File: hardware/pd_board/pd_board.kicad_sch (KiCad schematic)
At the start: 48 parts, among them J1 USB_C_Receptacle_USB2.0_16P, J2 CC1_TP, J3 CC2_TP, J4 Debug Port, J5 UART_Port, J6 VBUS_JP, J7 VCONN_JP, J8 VIN_ENA_JP, U1 FUSB302BMPX, U2 TPS5420D, U3 STM32F072CBUx

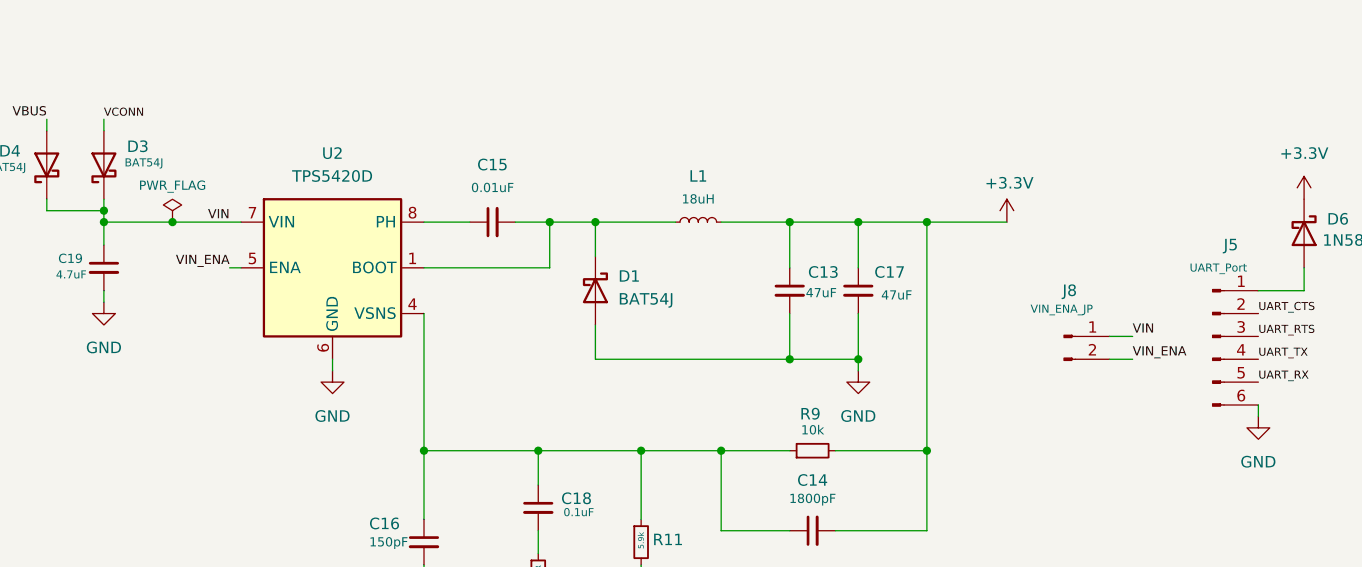
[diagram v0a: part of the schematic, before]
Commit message: update
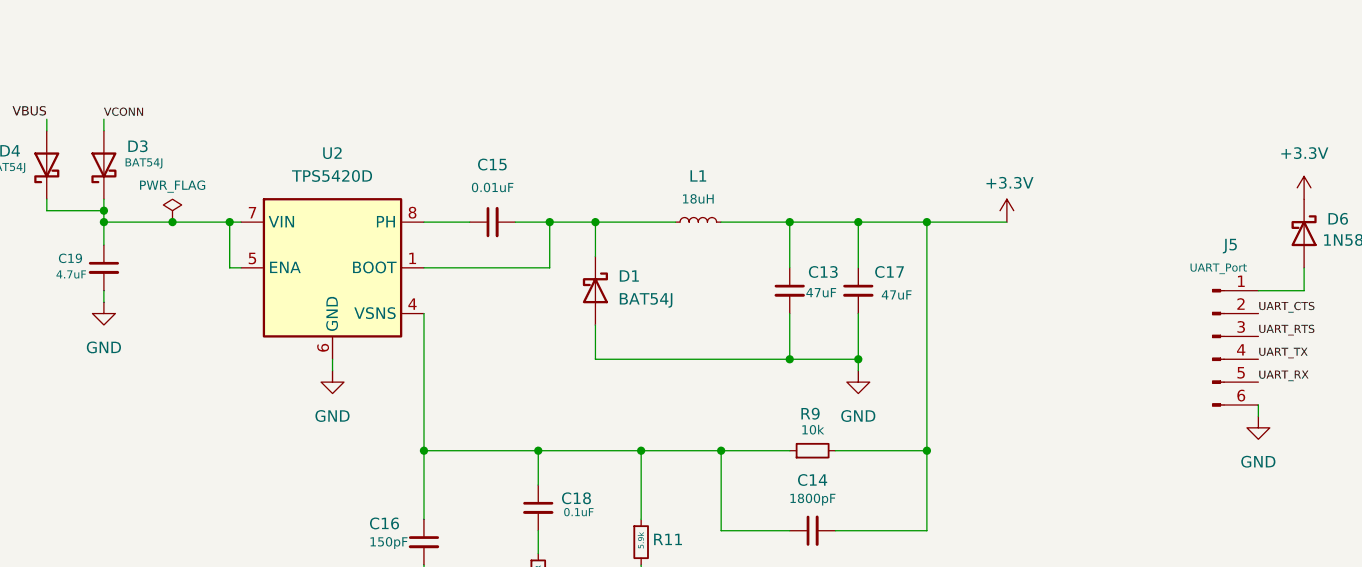
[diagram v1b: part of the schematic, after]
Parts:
- removed J8: VIN_ENA_JP, Connector_PinHeader_2.54mm:PinHeader_1x02_P2.54mm_Vertical, symbol Connector:Conn_01x02_Pin
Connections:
- net VIN_ENA is gone; now on an unnamed net: U2.5 (ENA)
- net VIN: no longer names the net of C19.1, D3.1 (K), D4.1 (K), U2.7 (VIN)

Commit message: update
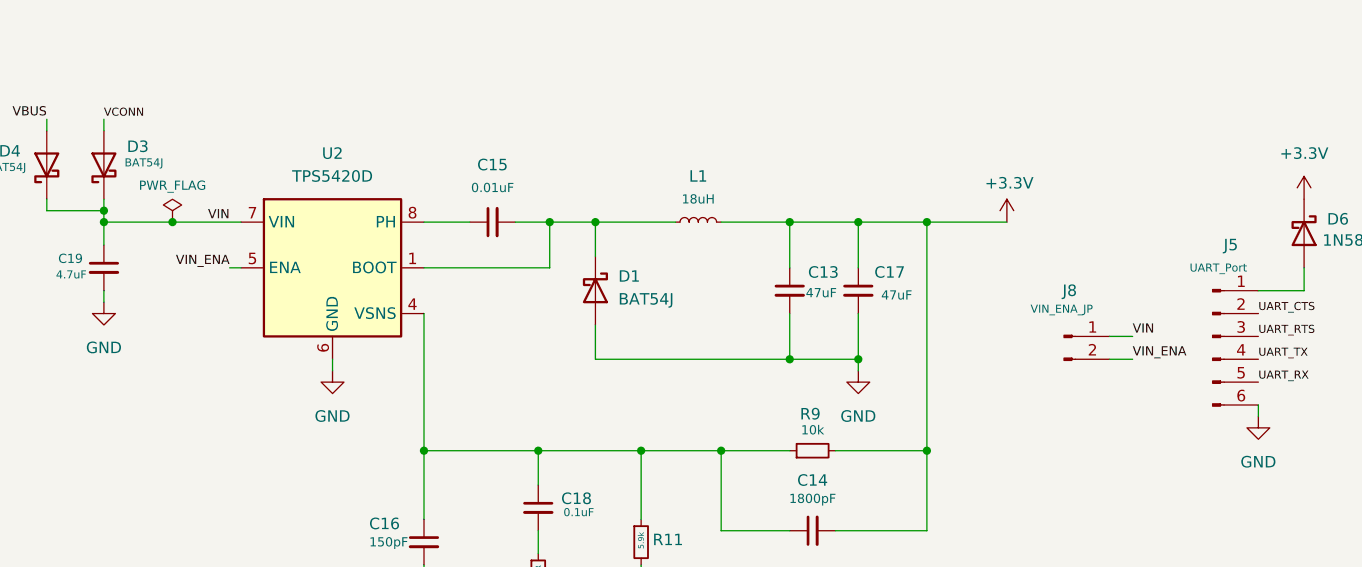
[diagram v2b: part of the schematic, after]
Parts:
- added J8: VIN_ENA_JP, Connector_PinHeader_2.54mm:PinHeader_1x02_P2.54mm_Vertical, symbol Connector:Conn_01x02_Pin
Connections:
- net VIN: now reaches C19.1, D3.1 (K), D4.1 (K), U2.7 (VIN)
- net VIN: now also J8.1 (Pin_1); no longer U2.5 (ENA)
- new net VIN_ENA: J8.2 (Pin_2), U2.5 (ENA)
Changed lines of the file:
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@@
-	)
-	(junction
-		(at 48.26 121.92)
-		(diameter 0)
-		(color 0 0 0 0)
 	)
 	(junction
@@
 	(wire
 		(pts
+			(xy 146.05 137.16) (xy 148.59 137.16)
+		)
+		(stroke
+			(width 0)
+			(type default)
+		)
+	)
+	(wire
+		(pts
 			(xy 27.94 110.49) (xy 27.94 111.76)
 		)
@@
 	(wire
 		(pts
-			(xy 48.26 121.92) (xy 49.53 121.92)
-		)
-		(stroke
-			(width 0)
-			(type default)
-		)
-	)
-	(wire
-		(pts
 			(xy 82.55 40.64) (xy 110.49 40.64)
 		)
@@
 	(wire
 		(pts
+			(xy 49.53 127) (xy 48.26 127)
+		)
+		(stroke
+			(width 0)
+			(type default)
+		)
+	)
+	(wire
+		(pts
 			(xy 175.26 27.94) (xy 177.8 27.94)
 		)
@@
 	(wire
 		(pts
-			(xy 48.26 127) (xy 48.26 121.92)
-		)
-		(stroke
-			(width 0)
-			(type default)
-		)
-	)
-	(wire
-		(pts
-			(xy 49.53 127) (xy 48.26 127)
-		)
-		(stroke
-			(width 0)
-			(type default)
-		)
-	)
-	(wire
-		(pts
 			(xy 82.55 167.64) (xy 93.98 167.64)
 		)
@@
 	(wire
 		(pts
+			(xy 146.05 134.62) (xy 148.59 134.62)
+		)
+		(stroke
+			(width 0)
+			(type default)
+		)
+	)
+	(wire
+		(pts
 			(xy 102.87 147.32) (xy 110.49 147.32)
 		)
@@
 	(wire
 		(pts
-			(xy 41.91 121.92) (xy 48.26 121.92)
+			(xy 41.91 121.92) (xy 49.53 121.92)
 		)
 		(stroke
@@
 		)
 	)
+	(label "VIN"
+		(at 148.59 134.62 0)
+		(effects
+			(font
+				(size 1.016 1.016)
+			)
+			(justify left bottom)
+		)
+	)
 	(label "I2C_SDA"
 		(at 205.74 95.25 180)
@@
 		)
 	)
+	(label "VIN"
+		(at 48.26 121.92 180)
+		(effects
+			(font
+				(size 1.016 1.016)
+			)
+			(justify right bottom)
+		)
+	)
 	(label "VBUS"
 		(at 27.94 110.49 180)
@@
 		)
 	)
+	(label "VIN_ENA"
+		(at 148.59 137.16 0)
+		(effects
+			(font
+				(size 1.016 1.016)
+			)
+			(justify left bottom)
+		)
+	)
 	(label "VBUS"
 		(at 111.76 36.83 0)
@@
 			)
 			(justify left bottom)
+		)
+	)
+	(label "VIN_ENA"
+		(at 48.26 127 180)
+		(effects
+			(font
+				(size 1.016 1.016)
+			)
+			(justify right bottom)
 		)
 	)
@@
 					(unit 1)
 				)
+			)
+		)
+	)
+	(symbol
+		(lib_id "Connector:Conn_01x02_Pin")
+		(at 140.97 134.62 0)
+		(unit 1)
+		(exclude_from_sim no)
+		(in_bom yes)
+		(on_board yes)
+		(dnp no)
+		(property "Reference" "J8"
+			(at 141.605 129.54 0)
+			(effects
+				(font
+					(size 1.27 1.27)
+				)
+			)
+		)
+		(property "Value" "VIN_ENA_JP"
+			(at 140.716 131.572 0)
+			(effects
+				(font
+					(size 0.889 0.889)
+				)
+			)
+		)
+		(property "Footprint" "Connector_PinHeader_2.54mm:PinHeader_1x02_P2.54mm_Vertical"
+			(at 140.97 134.62 0)
+			(effects
+				(font
+					(size 1.27 1.27)
+				)
+				(hide yes)
+			)
+		)
+		(property "Datasheet" "~"
+			(at 140.97 134.62 0)
+			(effects
+				(font
+					(size 1.27 1.27)
+				)
+				(hide yes)
+			)
+		)
+		(property "Description" "Generic connector, single row, 01x02, script generated"
+			(at 140.97 134.62 0)
+			(effects
+				(font
+					(size 1.27 1.27)
+				)
+				(hide yes)
+			)
+		)
+		(pin "1"
+		)
+		(pin "2"
+		)
+		(instances
+			(project ""
+				(path "/9d05689f-cd28-4719-8892-8398308a18b8"
+					(reference "J8")
+					(unit 1)
+				)
